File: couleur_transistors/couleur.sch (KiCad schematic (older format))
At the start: 17 parts, among them P1 CONN_02X03, P2 Mounting, Q1 Q_PNP_BEC, Q2 Q_PNP_BEC, Q3 Q_PNP_BEC, U1 S4282-51

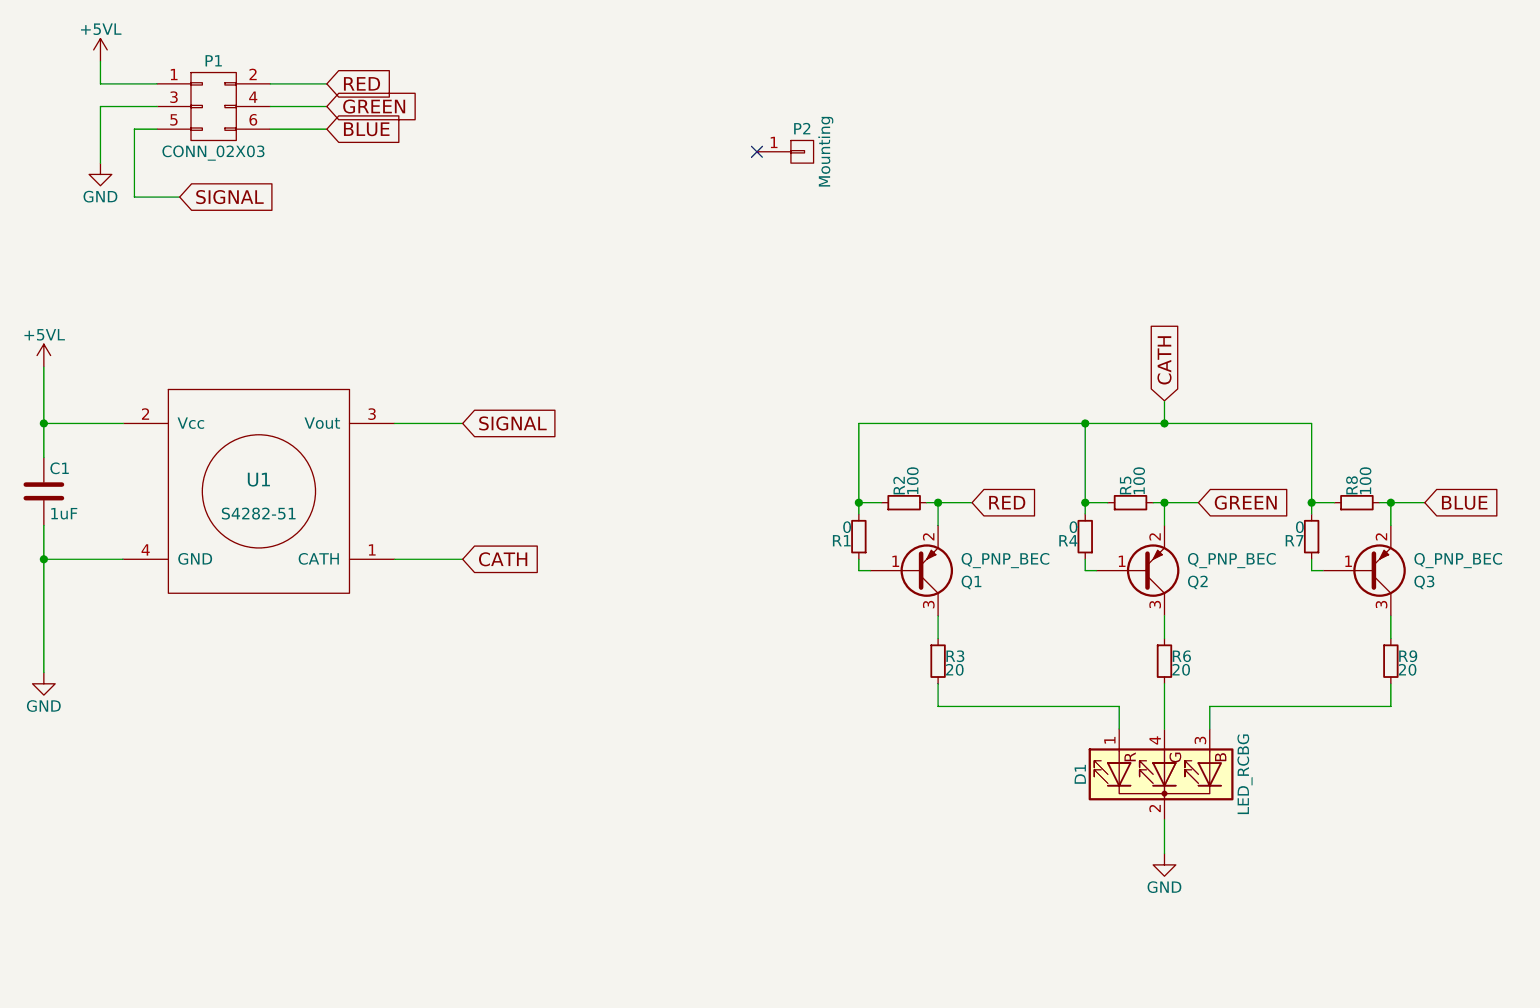
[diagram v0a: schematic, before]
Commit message: Couleur
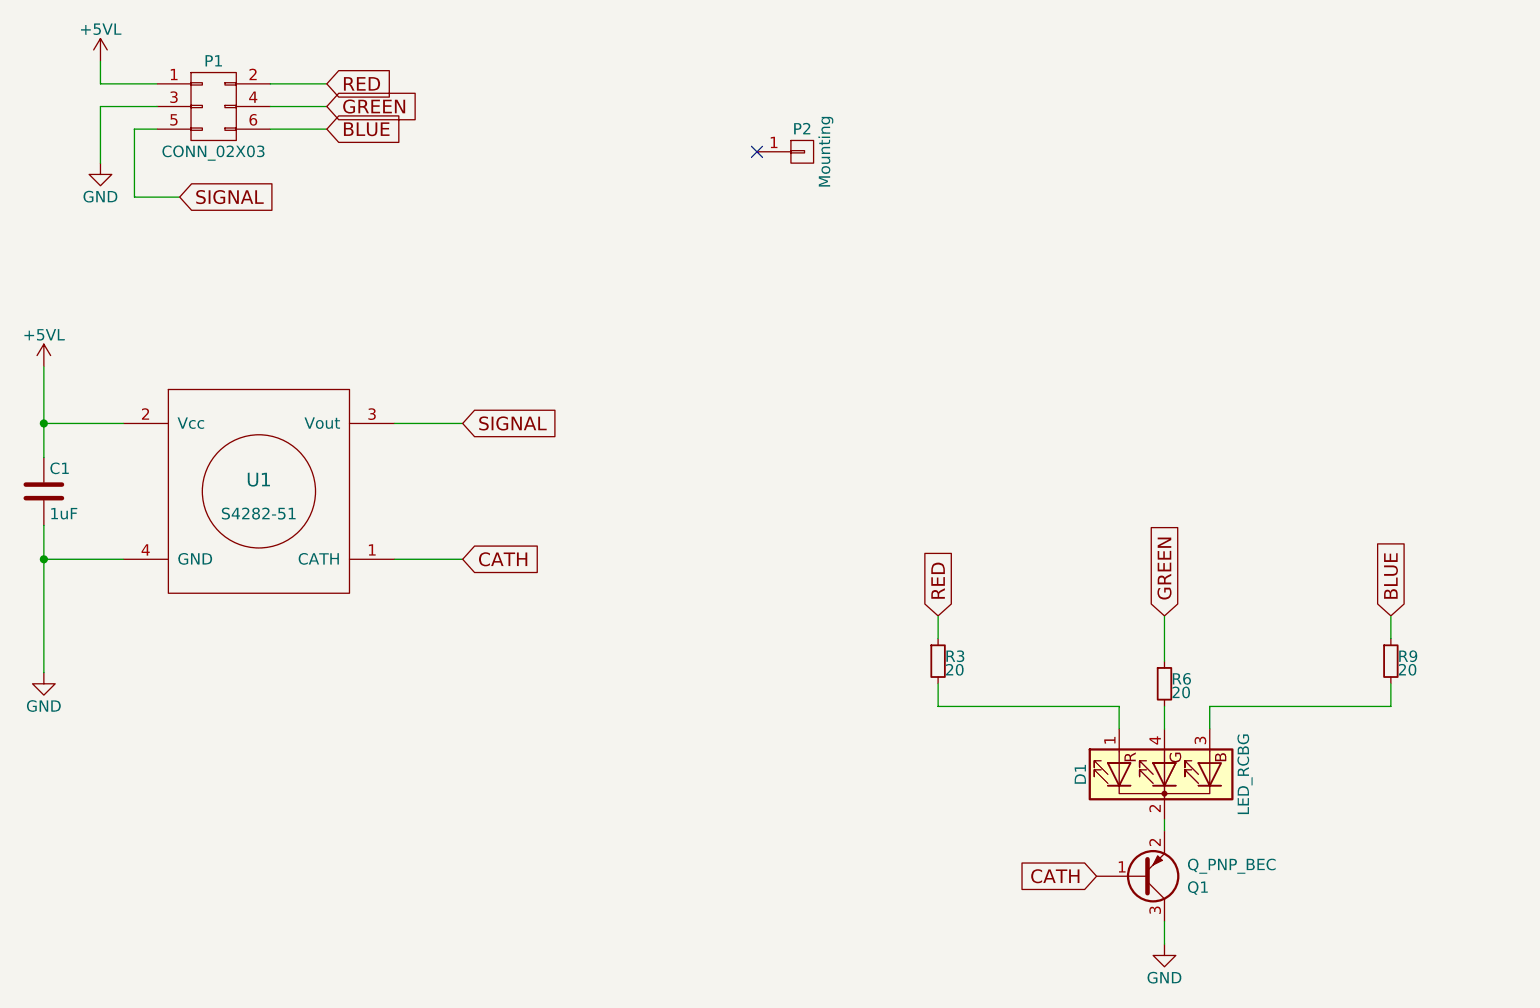
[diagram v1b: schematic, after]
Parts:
- removed Q2, Q3: Q_PNP_BEC, TO_SOT_Packages_SMD:SOT-23, symbol Q_PNP_BEC
- removed R1, R4, R7: 0, Resistors_SMD:R_0603_HandSoldering, symbol R_Small
- removed R2, R5, R8: 100, Resistors_SMD:R_0603_HandSoldering, symbol R_Small
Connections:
- net BLUE: now also R9.1
- net CATH: now also Q1.1 (B)
- net GND: now also Q1.3 (C); no longer D1.2 (K)
- net GREEN: now also R6.1
- net RED: now also R3.1; no longer Q1.2 (E)
- new net: D1.2 (K), Q1.2 (E)
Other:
- moved on the sheet: Q1, R6
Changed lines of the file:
@@
 Wire Wire Line
 	5400 3700 5100 3700
-Text GLabel 7650 4050 2    60   Input ~ 0
+Text GLabel 7500 4550 1    60   Input ~ 0
 RED
-Text GLabel 8650 4050 2    60   Input ~ 0
+Text GLabel 8500 4550 1    60   Input ~ 0
 GREEN
-Text GLabel 9650 4050 2    60   Input ~ 0
+Text GLabel 9500 4550 1    60   Input ~ 0
 BLUE
 $Comp
@@
 L GND #PWR05
 U 1 1 5A7A0A21
-P 8500 5600
-F 0 "#PWR05" H 8500 5350 50  0001 C CNN
-F 1 "GND" H 8500 5450 50  0000 C CNN
-F 2 "" H 8500 5600 50  0000 C CNN
-F 3 "" H 8500 5600 50  0000 C CNN
-	1    8500 5600
+P 8500 6000
+F 0 "#PWR05" H 8500 5750 50  0001 C CNN
+F 1 "GND" H 8500 5850 50  0000 C CNN
+F 2 "" H 8500 6000 50  0000 C CNN
+F 3 "" H 8500 6000 50  0000 C CNN
+	1    8500 6000
 	1    0    0    -1
 $EndComp
-Wire Wire Line
-	8500 5450 8500 5600
 $Comp
 L Q_PNP_BEC Q1
 U 1 1 5A7A0A6A
-P 7400 4350
-F 0 "Q1" H 7600 4400 50  0000 L CNN
-F 1 "Q_PNP_BEC" H 7600 4300 50  0000 L CNN
-F 2 "TO_SOT_Packages_SMD:SOT-23" H 7600 4450 50  0001 C CNN
-F 3 "" H 7400 4350 50  0000 C CNN
-	1    7400 4350
+P 8400 5700
+F 0 "Q1" H 8600 5750 50  0000 L CNN
+F 1 "Q_PNP_BEC" H 8600 5650 50  0000 L CNN
+F 2 "TO_SOT_Packages_SMD:SOT-23" H 8600 5800 50  0001 C CNN
+F 3 "" H 8400 5700 50  0000 C CNN
+	1    8400 5700
 	1    0    0    1
 $EndComp
@@
 L R_Small R6
 U 1 1 5A7A0C7B
-P 8500 4750
-F 0 "R6" H 8530 4770 50  0000 L CNN
-F 1 "20" H 8530 4710 50  0000 L CNN
-F 2 "Resistors_SMD:R_0603_HandSoldering" H 8500 4750 50  0001 C CNN
-F 3 "" H 8500 4750 50  0000 C CNN
-	1    8500 4750
+P 8500 4850
+F 0 "R6" H 8530 4870 50  0000 L CNN
+F 1 "20" H 8530 4810 50  0000 L CNN
+F 2 "Resistors_SMD:R_0603_HandSoldering" H 8500 4850 50  0001 C CNN
+F 3 "" H 8500 4850 50  0000 C CNN
+	1    8500 4850
 	1    0    0    -1
 $EndComp
@@
 	1    0    0    -1
 $EndComp
-$Comp
-L R_Small R1
-U 1 1 5A7A0CF2
-P 7150 4200
-F 0 "R1" H 7180 4220 50  0000 L CNN
-F 1 "0" H 7180 4160 50  0000 L CNN
-F 2 "Resistors_SMD:R_0603_HandSoldering" H 7150 4200 50  0001 C CNN
-F 3 "" H 7150 4200 50  0000 C CNN
-	1    7150 4200
-	-1   0    0    1
-$EndComp
-$Comp
-L R_Small R2
-U 1 1 5A7A0D69
-P 7350 4050
-F 0 "R2" H 7380 4070 50  0000 L CNN
-F 1 "100" H 7380 4010 50  0000 L CNN
-F 2 "Resistors_SMD:R_0603_HandSoldering" H 7350 4050 50  0001 C CNN
-F 3 "" H 7350 4050 50  0000 C CNN
-	1    7350 4050
-	0    -1   -1   0
-$EndComp
 Text GLabel 5400 4300 2    60   Input ~ 0
 CATH
-Wire Wire Line
-	7200 4350 7150 4350
-Wire Wire Line
-	7150 4350 7150 4300
-Wire Wire Line
-	7500 4150 7500 4050
-Wire Wire Line
-	7450 4050 7650 4050
-Wire Wire Line
-	7250 4050 7150 4050
-Connection ~ 7500 4050
 Wire Wire Line
 	7500 4550 7500 4650
 Wire Wire Line
 	7500 4850 7500 4950
-Text GLabel 8500 3600 1    60   Input ~ 0
+Text GLabel 8200 5700 0    60   Input ~ 0
 CATH
-$Comp
-L R_Small R4
-U 1 1 5A7A1702
-P 8150 4200
-F 0 "R4" H 8180 4220 50  0000 L CNN
-F 1 "0" H 8180 4160 50  0000 L CNN
-F 2 "Resistors_SMD:R_0603_HandSoldering" H 8150 4200 50  0001 C CNN
-F 3 "" H 8150 4200 50  0000 C CNN
-	1    8150 4200
-	-1   0    0    1
-$EndComp
 Wire Wire Line
-	8150 3700 8150 4100
-$Comp
-L R_Small R5
-U 1 1 5A7A184F
-P 8350 4050
-F 0 "R5" H 8380 4070 50  0000 L CNN
-F 1 "100" H 8380 4010 50  0000 L CNN
-F 2 "Resistors_SMD:R_0603_HandSoldering" H 8350 4050 50  0001 C CNN
-F 3 "" H 8350 4050 50  0000 C CNN
-	1    8350 4050
-	0    -1   -1   0
-$EndComp
-Wire Wire Line
-	8250 4050 8150 4050
-Connection ~ 8150 4050
-$Comp
-L Q_PNP_BEC Q2
-U 1 1 5A7A18E8
-P 8400 4350
-F 0 "Q2" H 8600 4400 50  0000 L CNN
-F 1 "Q_PNP_BEC" H 8600 4300 50  0000 L CNN
-F 2 "TO_SOT_Packages_SMD:SOT-23" H 8600 4450 50  0001 C CNN
-F 3 "" H 8400 4350 50  0000 C CNN
-	1    8400 4350
-	1    0    0    1
-$EndComp
-Wire Wire Line
-	8150 4300 8150 4350
-Wire Wire Line
-	8150 4350 8200 4350
-Wire Wire Line
-	8450 4050 8650 4050
-Wire Wire Line
-	8500 4050 8500 4150
-Connection ~ 8500 4050
-Wire Wire Line
-	8500 4550 8500 4650
-Wire Wire Line
-	7150 3700 7150 4100
-Wire Wire Line
-	7150 3700 9150 3700
-Wire Wire Line
-	8500 3700 8500 3600
-Connection ~ 7150 4050
-Connection ~ 8150 3700
-$Comp
-L R_Small R7
-U 1 1 5A7A1EB9
-P 9150 4200
-F 0 "R7" H 9180 4220 50  0000 L CNN
-F 1 "0" H 9180 4160 50  0000 L CNN
-F 2 "Resistors_SMD:R_0603_HandSoldering" H 9150 4200 50  0001 C CNN
-F 3 "" H 9150 4200 50  0000 C CNN
-	1    9150 4200
-	-1   0    0    1
-$EndComp
-$Comp
-L R_Small R8
-U 1 1 5A7A1F6E
-P 9350 4050
-F 0 "R8" H 9380 4070 50  0000 L CNN
-F 1 "100" H 9380 4010 50  0000 L CNN
-F 2 "Resistors_SMD:R_0603_HandSoldering" H 9350 4050 50  0001 C CNN
-F 3 "" H 9350 4050 50  0000 C CNN
-	1    9350 4050
-	0    -1   -1   0
-$EndComp
-Wire Wire Line
-	9150 3700 9150 4100
-Wire Wire Line
-	9150 4050 9250 4050
-Connection ~ 8500 3700
-Connection ~ 9150 4050
-$Comp
-L Q_PNP_BEC Q3
-U 1 1 5A7A20CB
-P 9400 4350
-F 0 "Q3" H 9600 4400 50  0000 L CNN
-F 1 "Q_PNP_BEC" H 9600 4300 50  0000 L CNN
-F 2 "TO_SOT_Packages_SMD:SOT-23" H 9600 4450 50  0001 C CNN
-F 3 "" H 9400 4350 50  0000 C CNN
-	1    9400 4350
-	1    0    0    1
-$EndComp
-Wire Wire Line
-	9450 4050 9650 4050
-Wire Wire Line
-	9500 4050 9500 4150
-Wire Wire Line
-	9200 4350 9150 4350
-Wire Wire Line
-	9150 4350 9150 4300
-Connection ~ 9500 4050
+	8500 4550 8500 4750
 Wire Wire Line
 	9500 4550 9500 4650
@@
 	8300 4950 8300 5050
 Wire Wire Line
-	8500 4850 8500 5050
+	8500 4950 8500 5050
 Wire Wire Line
 	9500 4850 9500 4950
@@
 Wire Wire Line
 	8700 4950 8700 5050
+Wire Wire Line
+	8500 5450 8500 5500
+Wire Wire Line
+	8500 5900 8500 6000
 $EndSCHEMATC

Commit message: maj
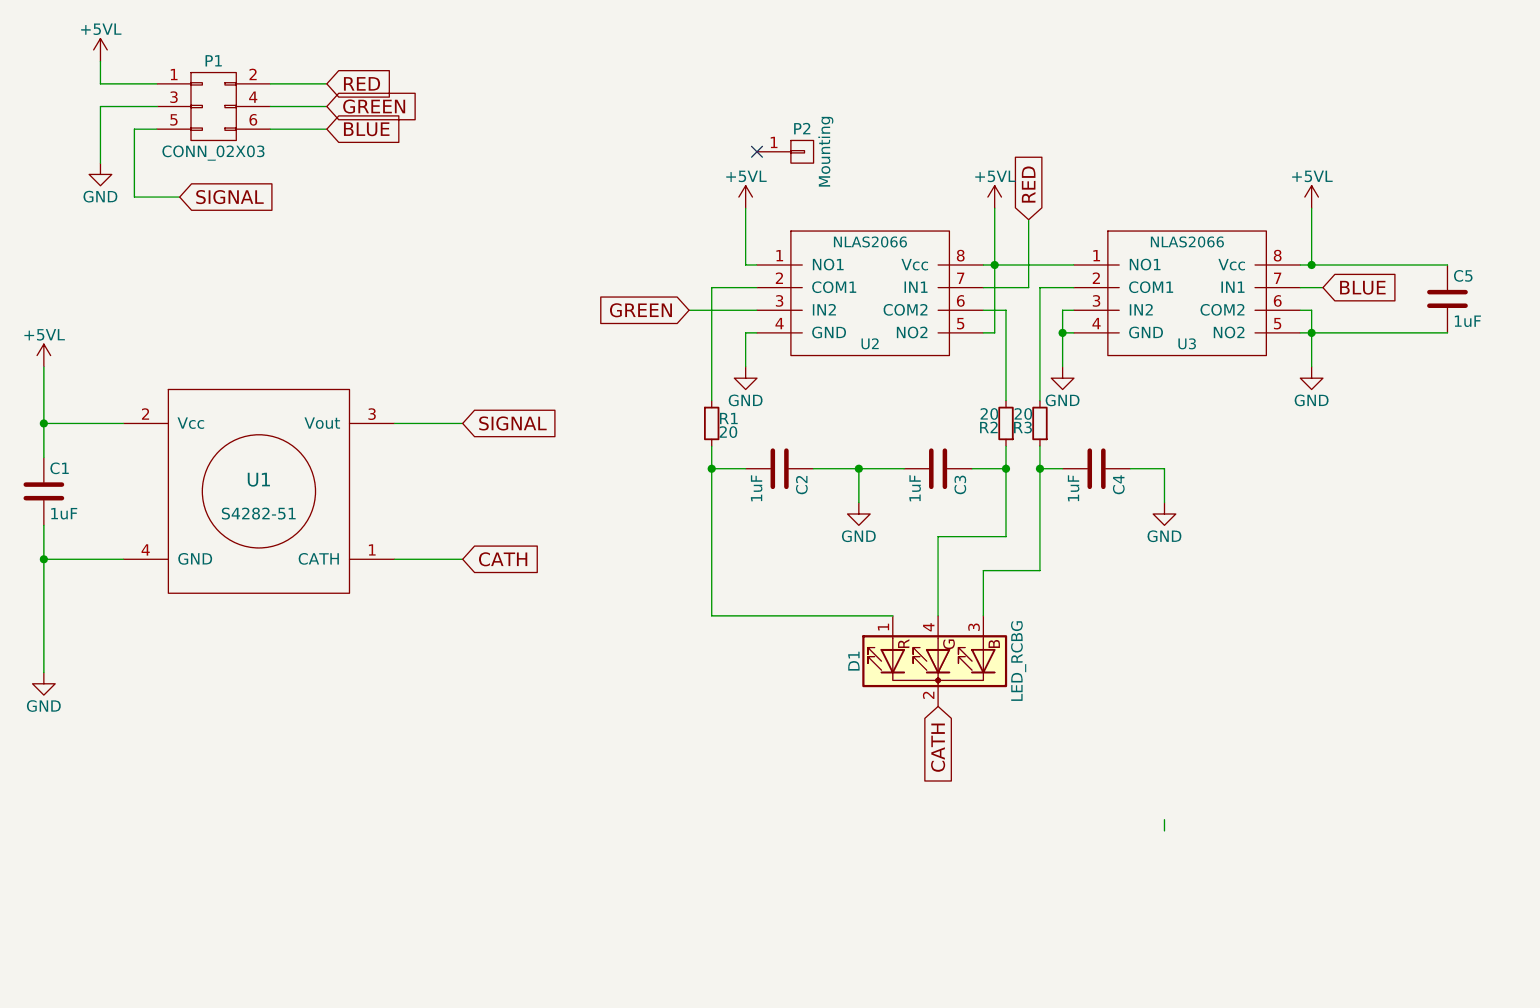
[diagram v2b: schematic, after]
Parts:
- removed Q1: Q_PNP_BEC, TO_SOT_Packages_SMD:SOT-23, symbol Q_PNP_BEC
- removed R6, R9: 20, Resistors_SMD:R_0603_HandSoldering, symbol R_Small
- added C2, C3, C4, C5: 1uF, Capacitors_SMD:C_0603_HandSoldering, symbol C
- added R1, R2: 20, Resistors_SMD:R_0603_HandSoldering, symbol R_Small
- added U2, U3: NLAS2066, Housings_SSOP:TSSOP-8_3x3mm_Pitch0.65mm, symbol NLAS2066
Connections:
- wire segments 28 -> 57
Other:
- moved on the sheet: D1
